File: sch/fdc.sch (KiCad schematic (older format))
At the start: 16 parts, among them X4 SLOT-34

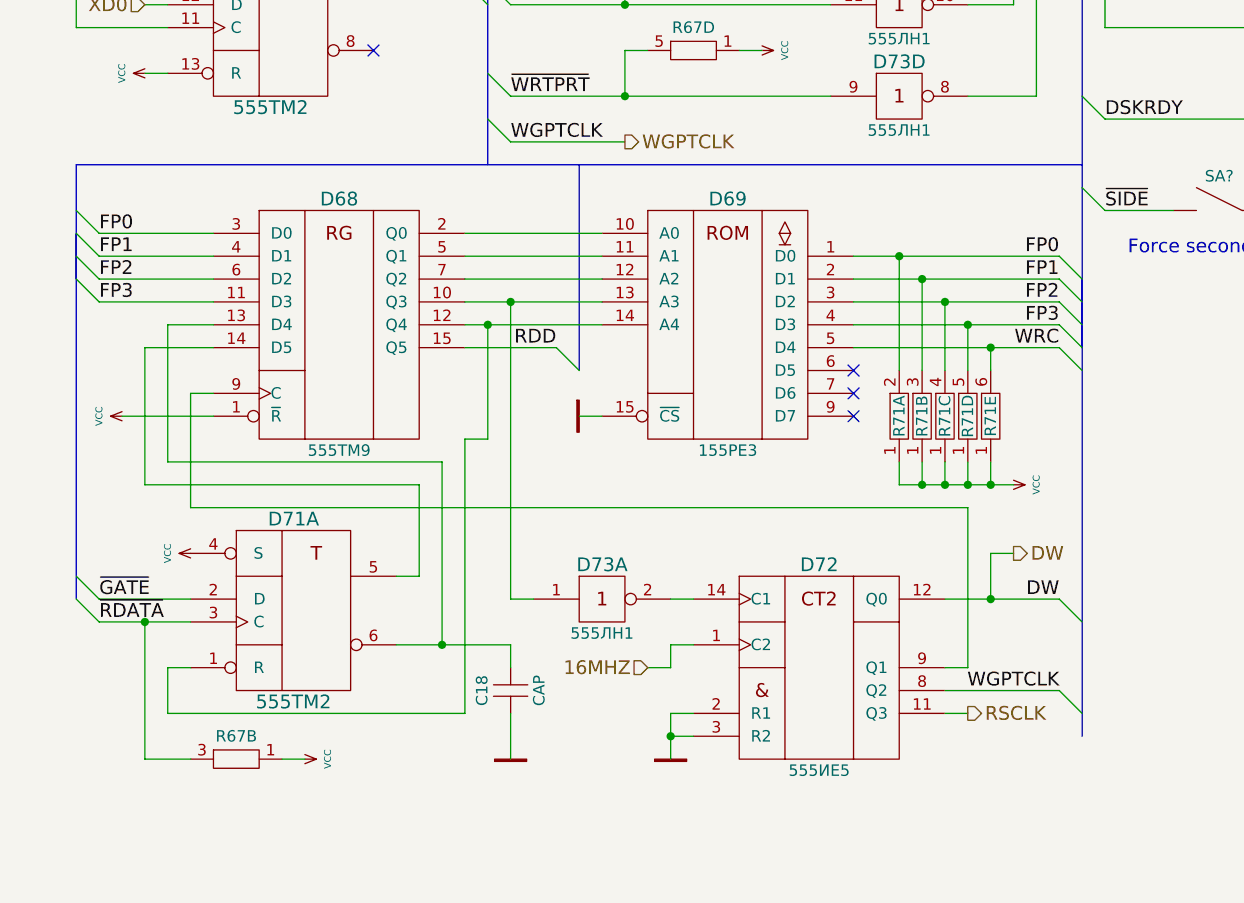
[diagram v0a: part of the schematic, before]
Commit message: GAL based PLL for FDC
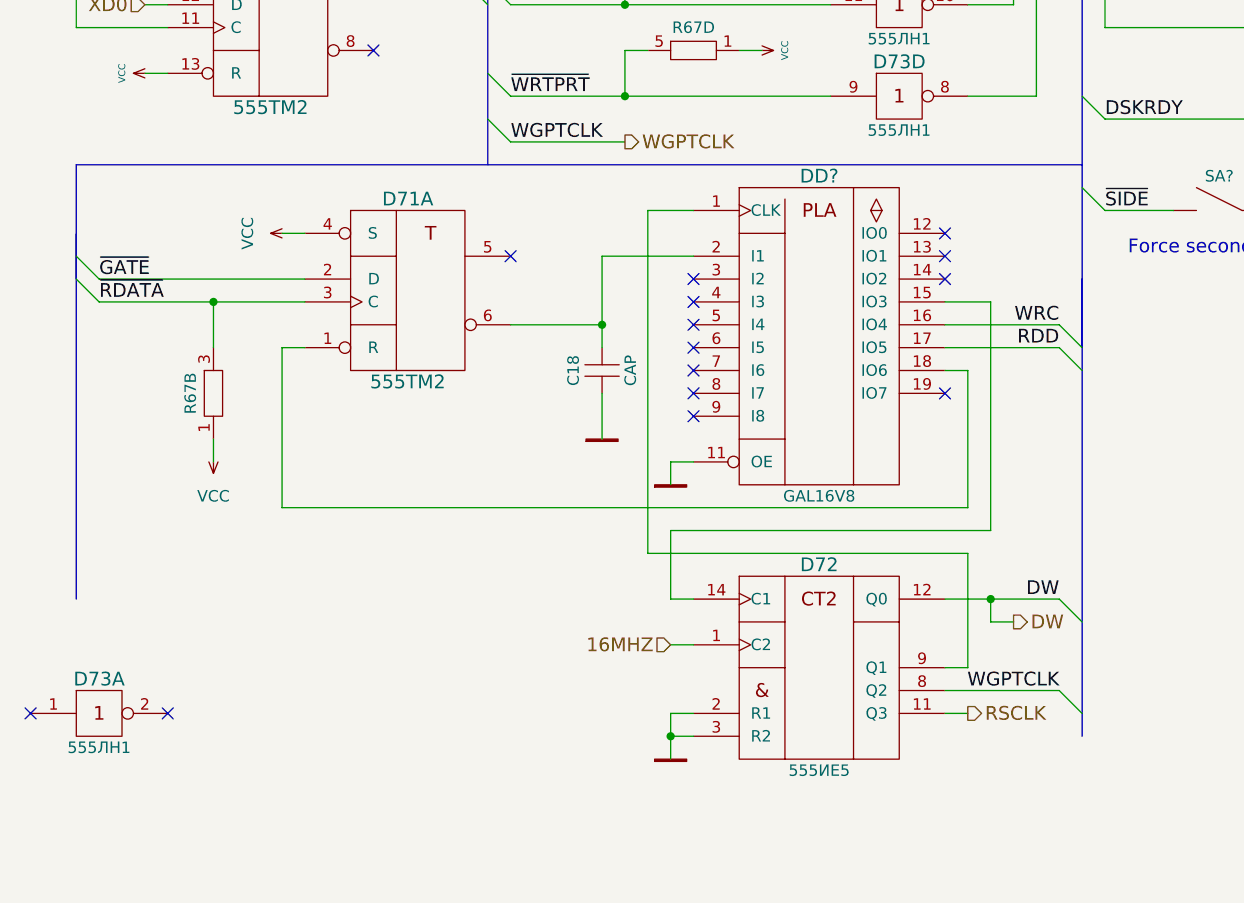
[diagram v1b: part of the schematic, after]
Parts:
- removed D68: 555ТМ9, MyLib:DIP-16, symbol 555ТМ9
- removed D69: 155РЕ3, MyLib:DIP-16, symbol 155РЕ3
- removed R71: RES_PACK8_C, MyLib:Resistor_Array_SIP5, symbol RES_PACK8_C
- added DD?: GAL16V8, symbol GAL16V8
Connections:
- net GND: now also DD?.10 (GND), DD?.11 (OE)
- net RDD: now also DD?.17 (IO5)
- net VCC: now also DD?.20 (VCC)
- net WRC: now also DD?.16 (IO4)
- net at D71.1 (R): now also DD?.18 (IO6)
- net at C18.2, D71.6: now also DD?.2 (I1)
- net at D72.9 (Q1): now also DD?.1 (CLK)
- net at D72.14 (C1): now also DD?.15 (IO3); no longer D73.2 (out)
- no-connect marks 20 -> 31
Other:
- moved on the sheet: C18, D71A, D73A, R67B
